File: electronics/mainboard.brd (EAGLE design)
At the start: 170 x 170 mm, 84 parts, among them T1 NPN_BC817,215, T2 NPN_BC817,215, T3 NPN_BC817,215, U1 CD4051BM, X1 JST-XH-10-PIN-LONG-PAD, X2 JST-XH-10-PIN-LONG-PAD, X3 JST-XH-10-PIN-LONG-PAD, X4 JST-XH-10-PIN-LONG-PAD, X5 JST-XH-10-PIN-LONG-PAD

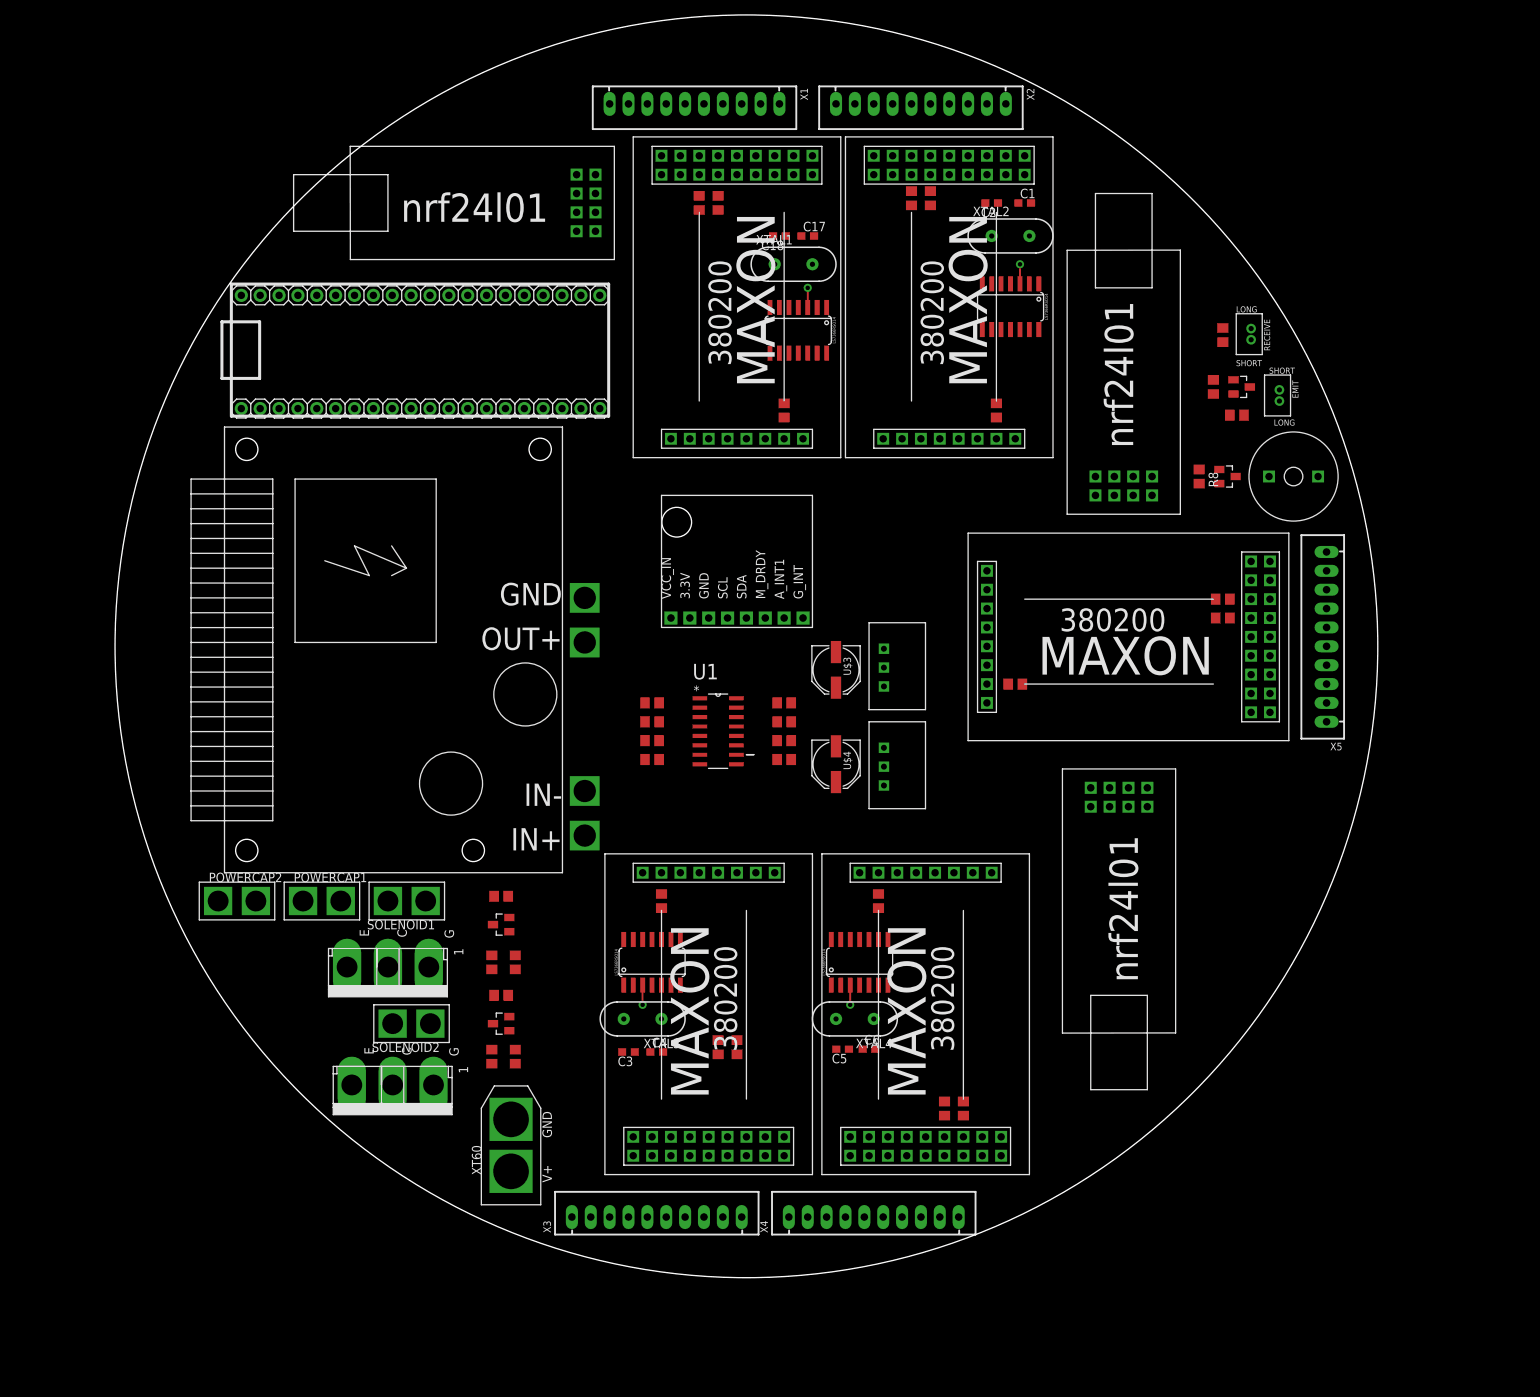
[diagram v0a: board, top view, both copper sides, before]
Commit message: SSL mainboard wip
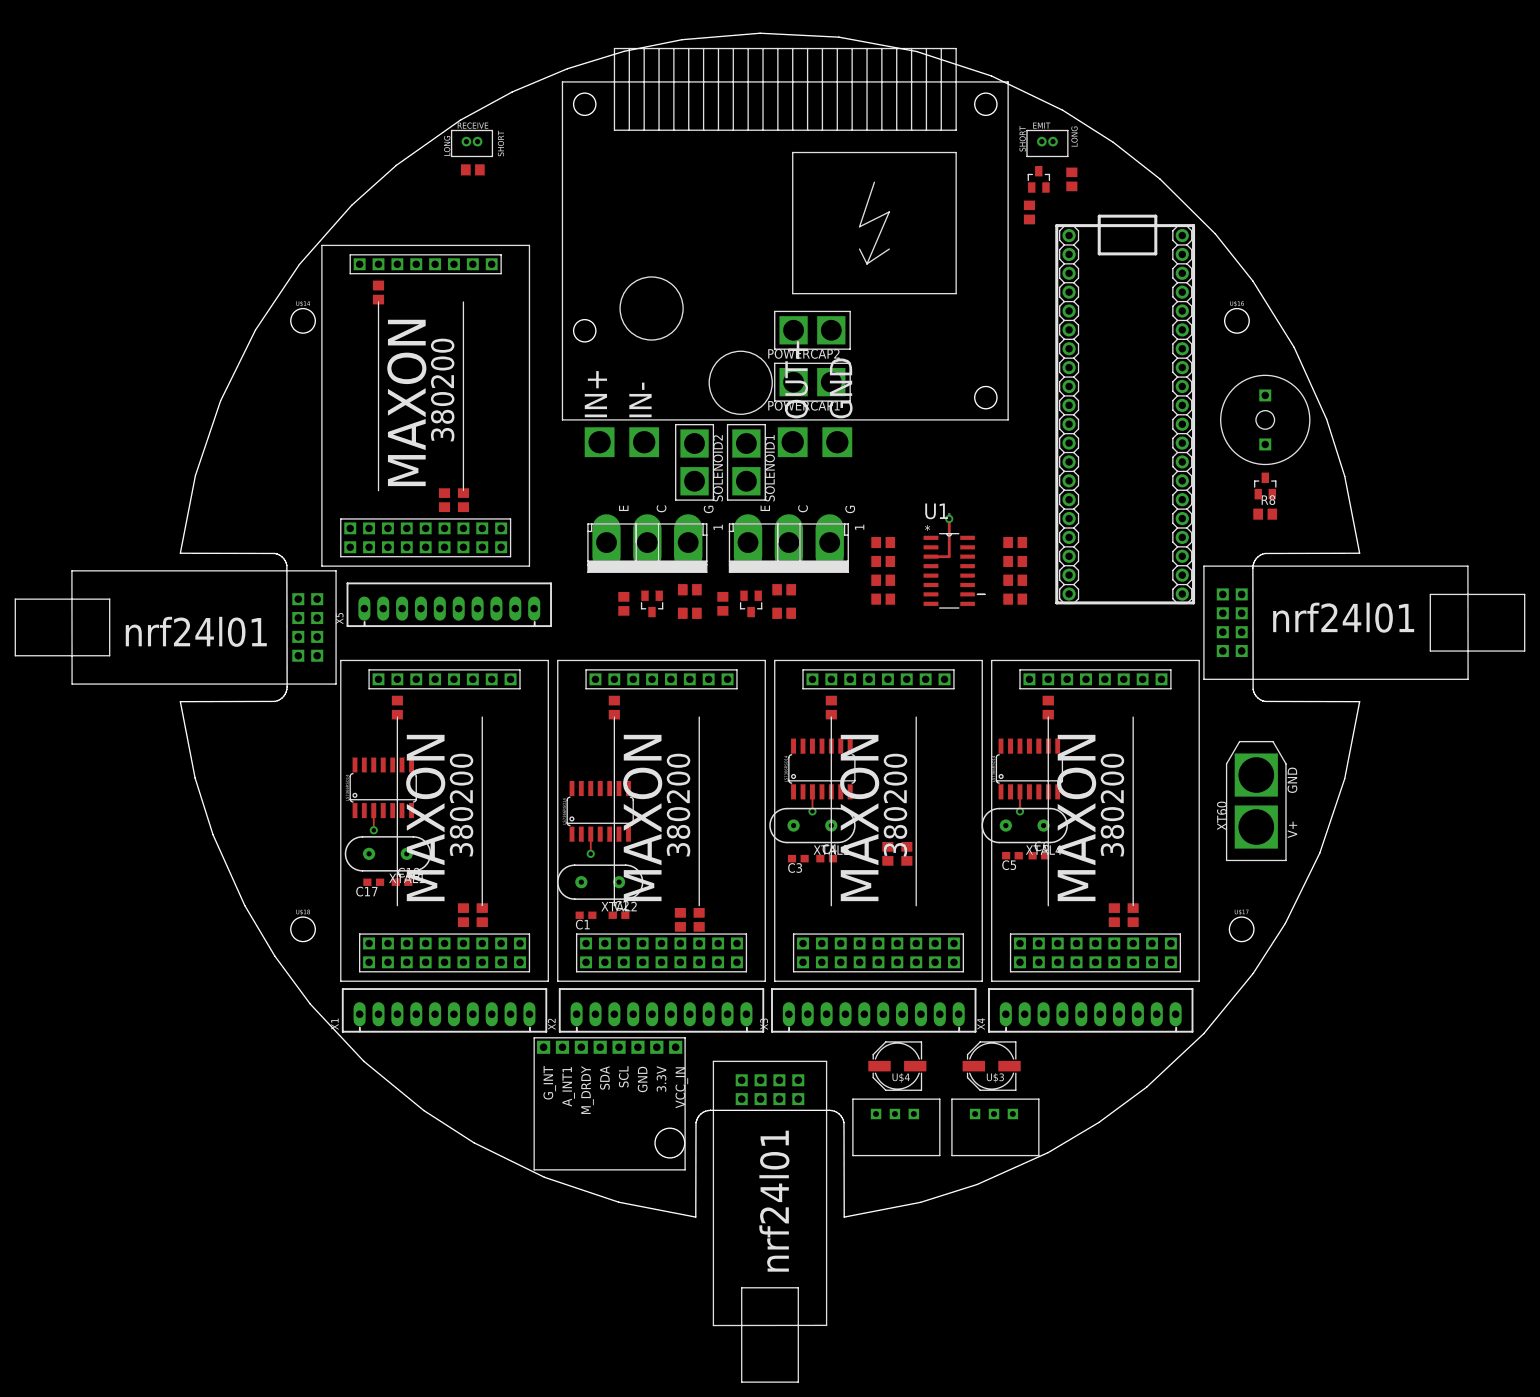
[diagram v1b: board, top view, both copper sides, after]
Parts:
- added U$14, U$16, U$17, U$18: (no value), SparkFun-Hardware:STAND-OFF
- moved X2 127.4 mm to (-11.4, -49.5), turned to 0 degrees
- moved X1 127.1 mm to (-40.6, -49.5), turned to 0 degrees
- moved MAPLE 126.9 mm to (58.7, 55.3), turned to 270 degrees
- moved X5 118.2 mm to (-40.0, 5.08), turned to 0 degrees
- moved POWERCAP2 112.8 mm to (11.4, 42.5), turned to 180 degrees
- moved C1 112.6 mm to (-21.6, -36.2), turned to 180 degrees
- moved XT60 110.5 mm to (72.6, -28.8)
- moved U$6 110.2 mm to (-30.5, -42.5), turned to 90 degrees
- moved U$7 110.1 mm to (-1.27, -42.5), turned to 90 degrees
- moved RECEIVE 108.4 mm to (-37.5, 67.9), turned to 0 degrees
- moved C2 108.2 mm to (-17.1, -36.2), turned to 0 degrees
- moved R29 106.0 mm to (-40.6, 19.7), turned to 90 degrees
- moved C17 104.8 mm to (-50.2, -31.8), turned to 180 degrees
- moved U$10 103.5 mm to (-33.0, 13.3), turned to 90 degrees
- moved R6 103.4 mm to (-36.8, 64.1), turned to 0 degrees
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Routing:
- net GND: track 10.6 -> 18.7 mm, vias 4 -> 5
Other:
- board size 170 x 170 mm -> 158.8 x 159.4 mm
